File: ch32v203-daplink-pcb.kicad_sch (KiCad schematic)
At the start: 26 parts, among them J1 USB2.0_C_v3, J2 DAPLink-SWD-Send-6Pin, J3 DAPLink-SWD-Send-10Pin, SW1 SW_SPDT, U1 STM32V103C8T6, U2 AMS1117-3.3, Y1 8M

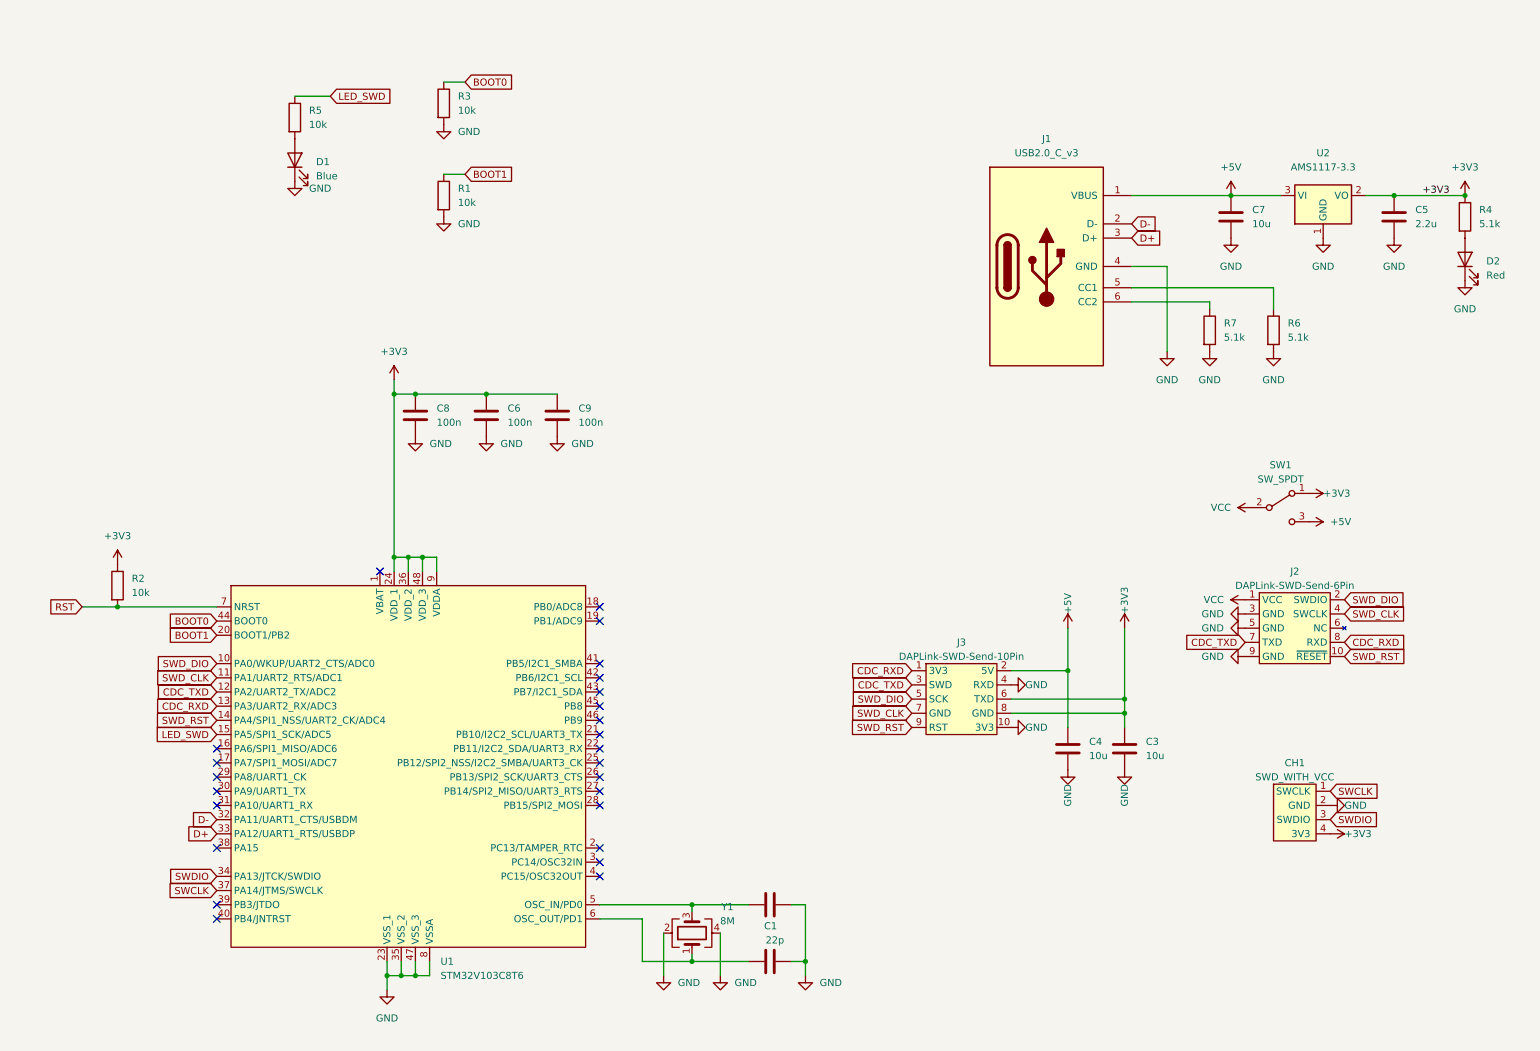
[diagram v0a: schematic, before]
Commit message: fix semantics
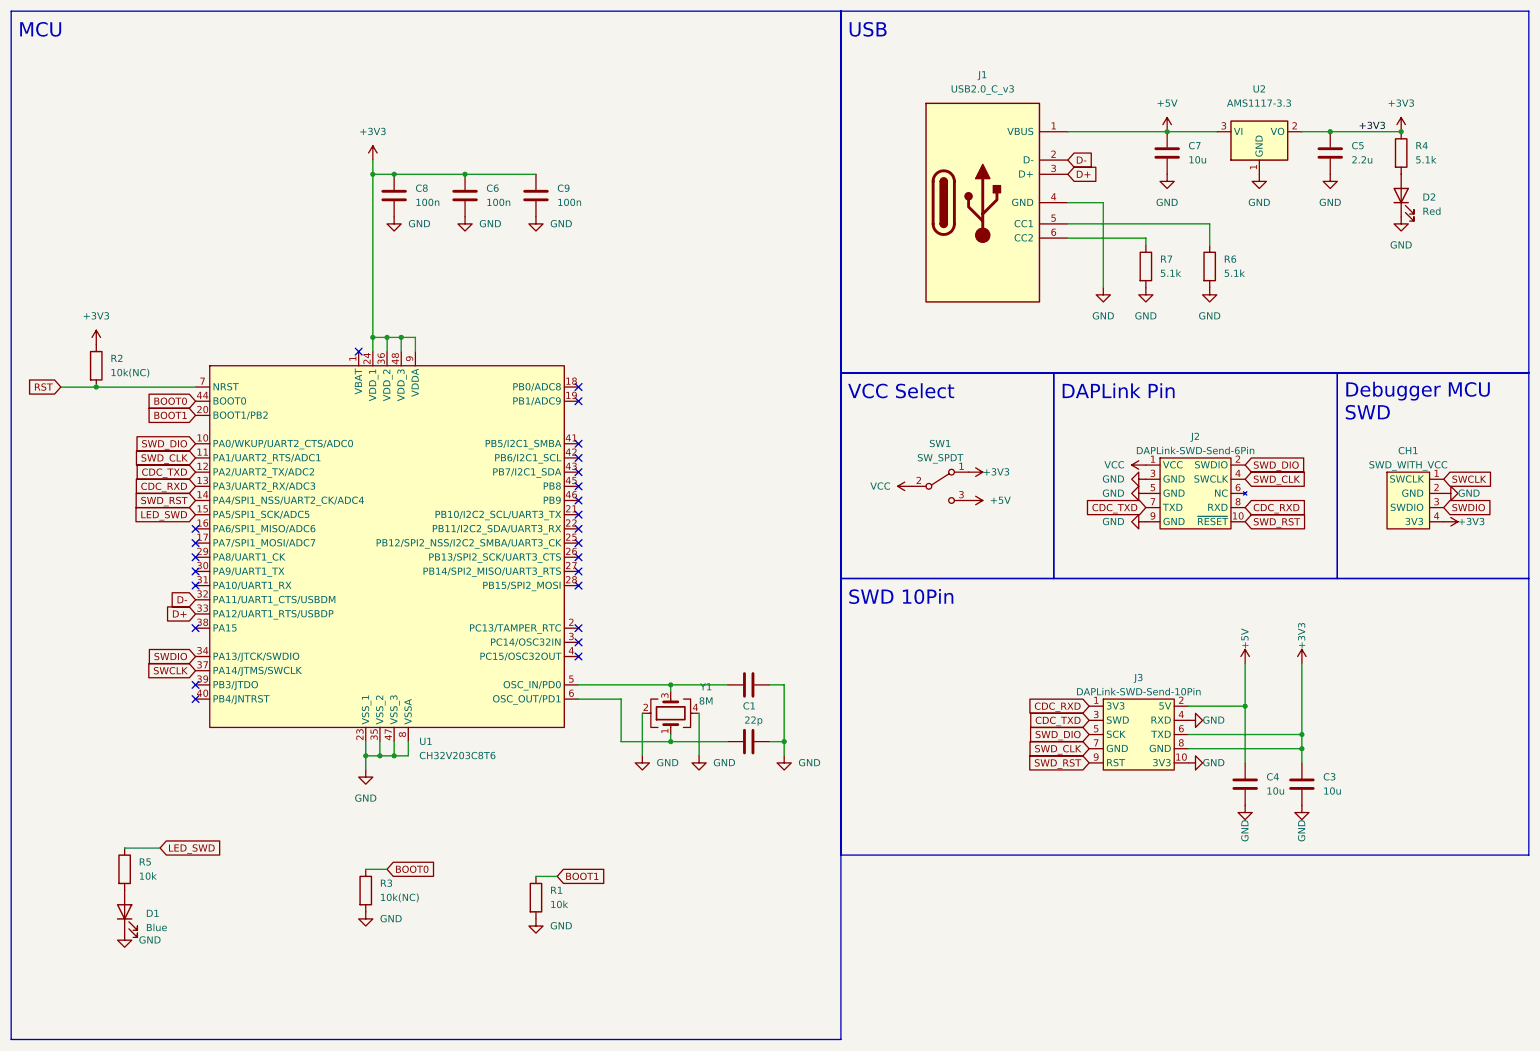
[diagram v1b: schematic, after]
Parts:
- R2, R3: value 10k -> 10k(NC)
- U1: value STM32V103C8T6 -> CH32V203C8T6
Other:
- note added: "DAPLink Pin"
- note added: "Debugger MCU SWD"
- note added: "MCU"
- note added: "SWD 10Pin"
- note added: "USB"
- note added: "VCC Select"
- title: (none) -> CH32V203 DapLink
- moved on the sheet: C1, C3, C4, C5, C6, C7, C8, C9, CH1, D1, D2, J1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
